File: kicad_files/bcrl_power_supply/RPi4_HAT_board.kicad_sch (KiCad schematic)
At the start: 6 parts

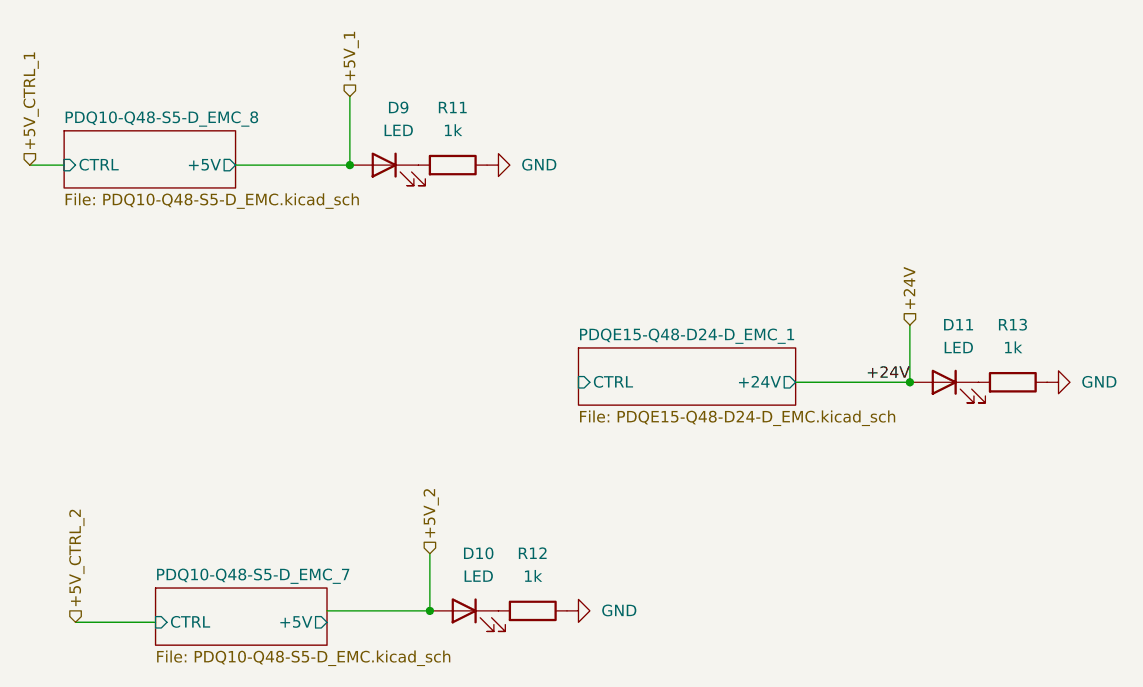
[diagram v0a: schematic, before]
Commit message: big changes
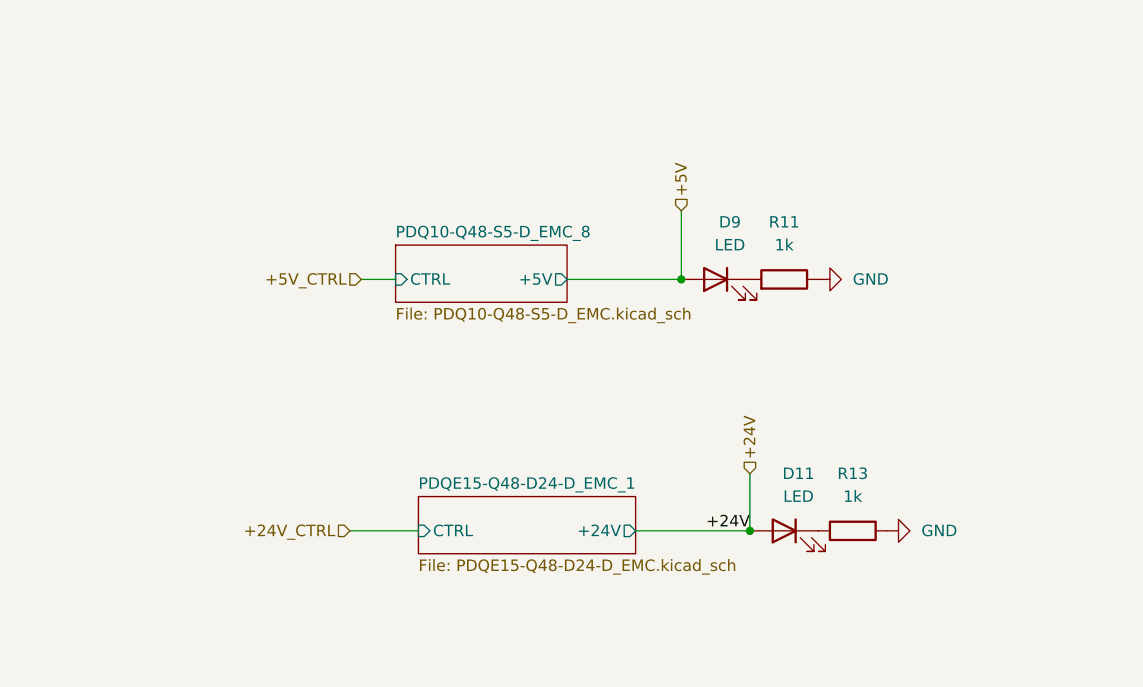
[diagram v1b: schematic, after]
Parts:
- removed D10: LED, LED_SMD:LED_0603_1608Metric, symbol Device:LED
- removed R12: 1k, Resistor_SMD:R_0603_1608Metric, symbol Device:R
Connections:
- net +5V_1 renamed +5V
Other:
- removed sheet PDQ10-Q48-S5-D_EMC_7
- moved on the sheet: D11, D9, R11, R13
